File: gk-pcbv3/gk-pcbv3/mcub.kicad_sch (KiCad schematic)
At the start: 10 parts, among them U4 STM32H7S7L8H6H, Y1 24MHz

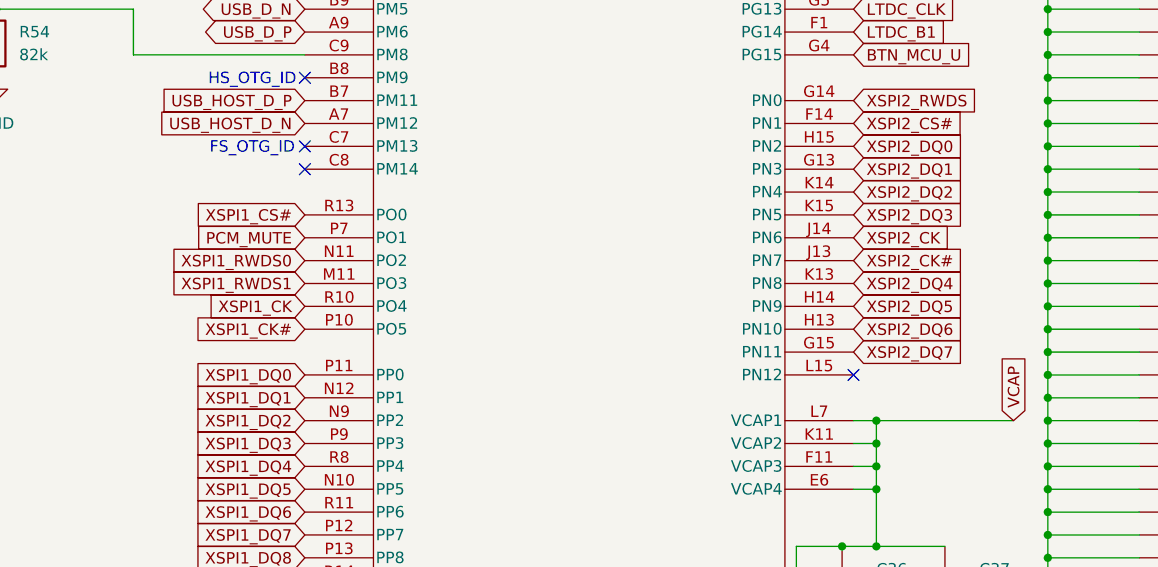
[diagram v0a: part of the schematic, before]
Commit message: hardware changes
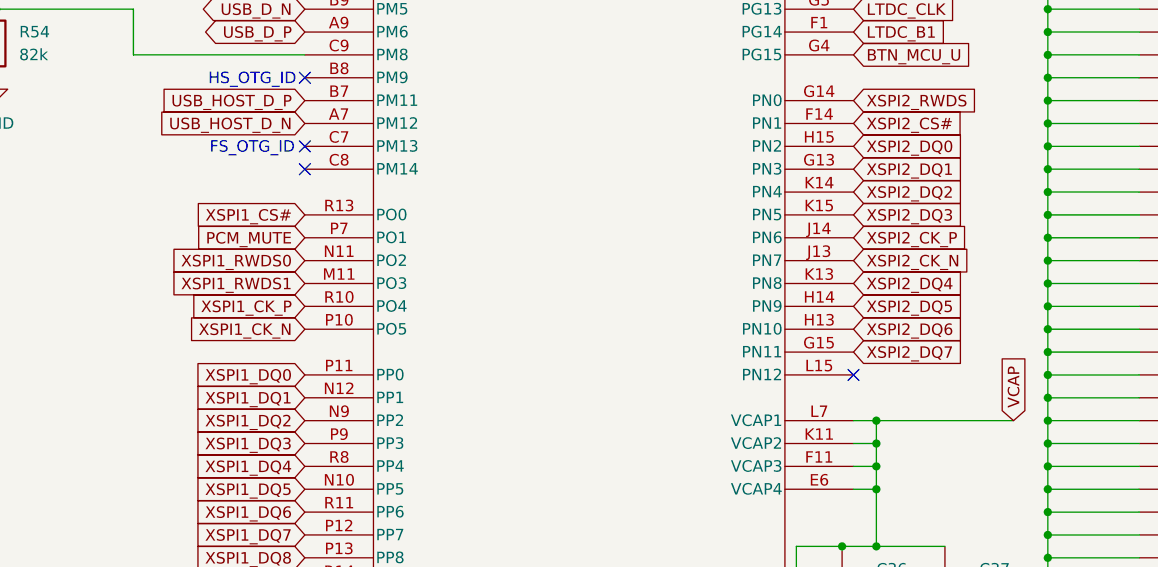
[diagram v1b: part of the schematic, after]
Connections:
- net XSPI1_CK renamed XSPI1_CK_P
- net XSPI1_CK# renamed XSPI1_CK_N
- net XSPI2_CK renamed XSPI2_CK_P
- net XSPI2_CK# renamed XSPI2_CK_N
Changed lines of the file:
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@@
 		)
 	)
-	(global_label "XSPI2_CK"
+	(global_label "XSPI2_CK_P"
 		(shape input)
 		(at 121.92 93.98 0)
@@
 		)
 		(property "Intersheetrefs" "${INTERSHEET_REFS}"
-			(at 133.9161 93.98 0)
+			(at 136.1537 93.98 0)
 			(effects
 				(font
@@
 		)
 	)
-	(global_label "XSPI1_CK#"
+	(global_label "XSPI1_CK_N"
 		(shape input)
 		(at 60.96 104.14 180)
@@
 		)
 		(property "Intersheetrefs" "${INTERSHEET_REFS}"
-			(at 47.6939 104.14 0)
+			(at 46.6658 104.14 0)
 			(effects
 				(font
@@
 		)
 	)
-	(global_label "XSPI1_CK"
+	(global_label "XSPI1_CK_P"
 		(shape input)
 		(at 60.96 101.6 180)
@@
 		)
 		(property "Intersheetrefs" "${INTERSHEET_REFS}"
-			(at 48.9639 101.6 0)
+			(at 46.7263 101.6 0)
 			(effects
 				(font
@@
 		)
 	)
-	(global_label "XSPI2_CK#"
+	(global_label "XSPI2_CK_N"
 		(shape input)
 		(at 121.92 96.52 0)
@@
 		)
 		(property "Intersheetrefs" "${INTERSHEET_REFS}"
-			(at 135.1861 96.52 0)
-			(effects
-				(font
+			(at 136.2142 96.52 0)
+			(effects
+				(font
